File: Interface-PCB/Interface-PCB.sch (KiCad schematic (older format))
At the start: 9 parts, among them J1 BARREL_JACK_PAD, J2 BARREL_JACK_PAD, J3 RASPBERRYPI-40-PIN-GPIO, J4 I2C_HEADER, M1 PERISTALTIC_PUMP, M2 PERISTALTIC_PUMP, M3 PERISTALTIC_PUMP, U1 TB6612FNG_BREAKOUT, U2 TB6612FNG_BREAKOUT

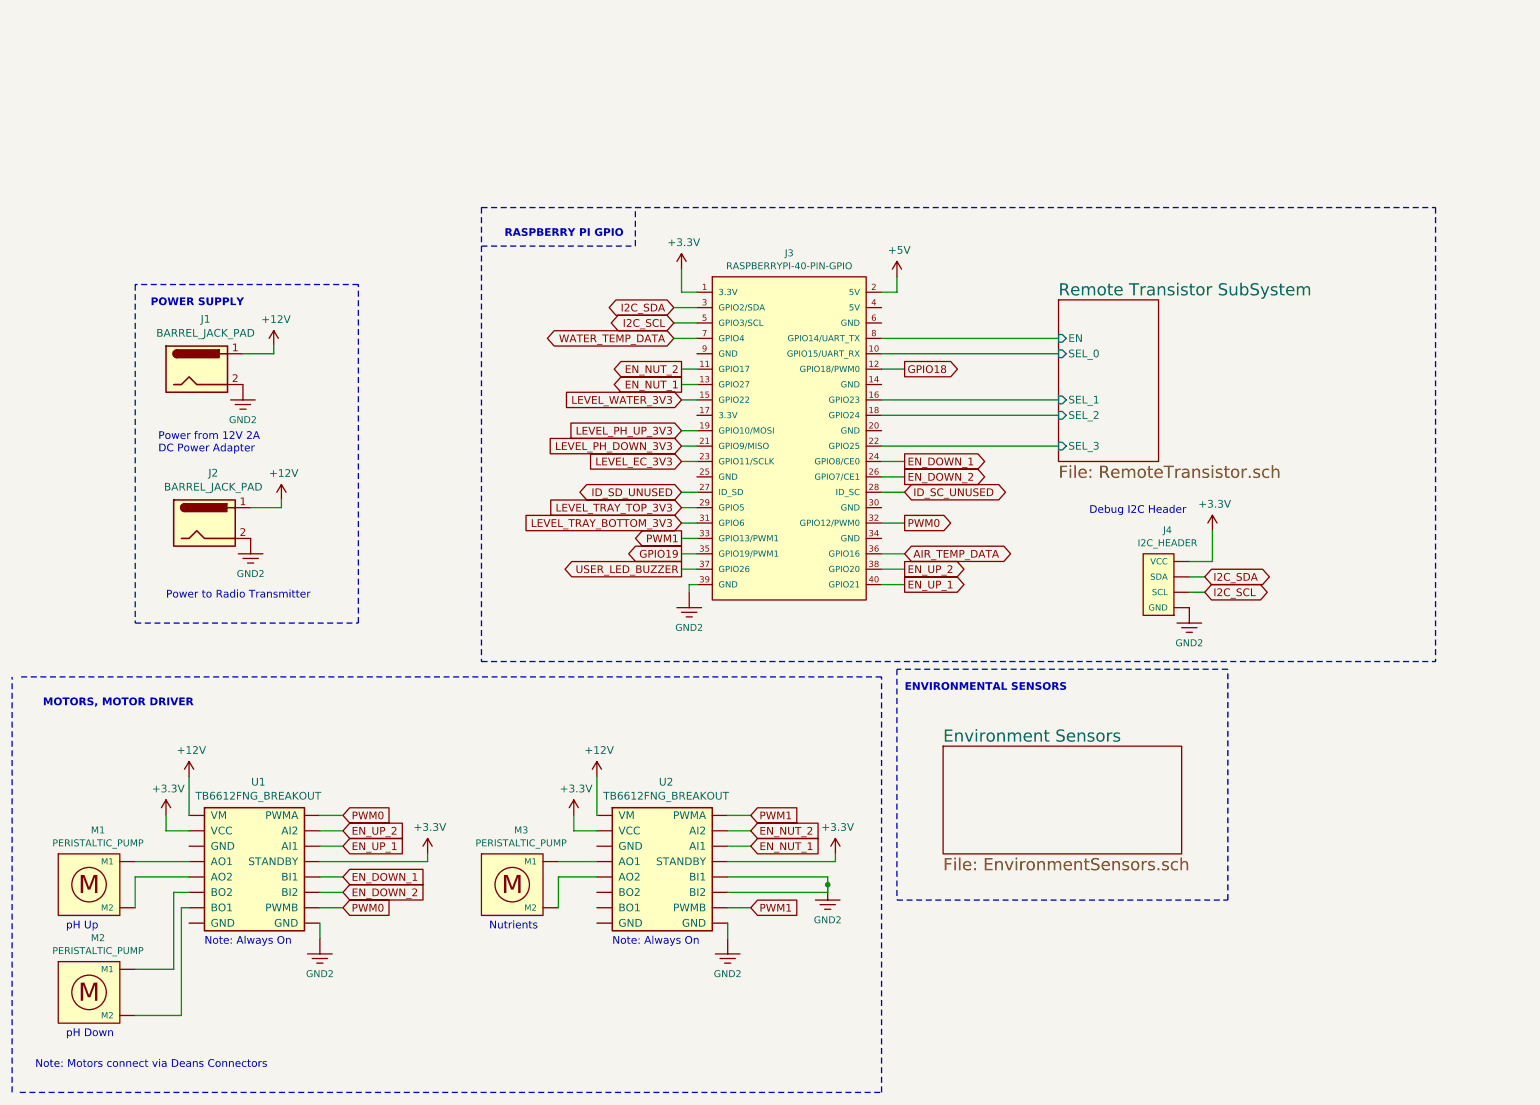
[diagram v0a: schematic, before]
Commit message: Review Schematic
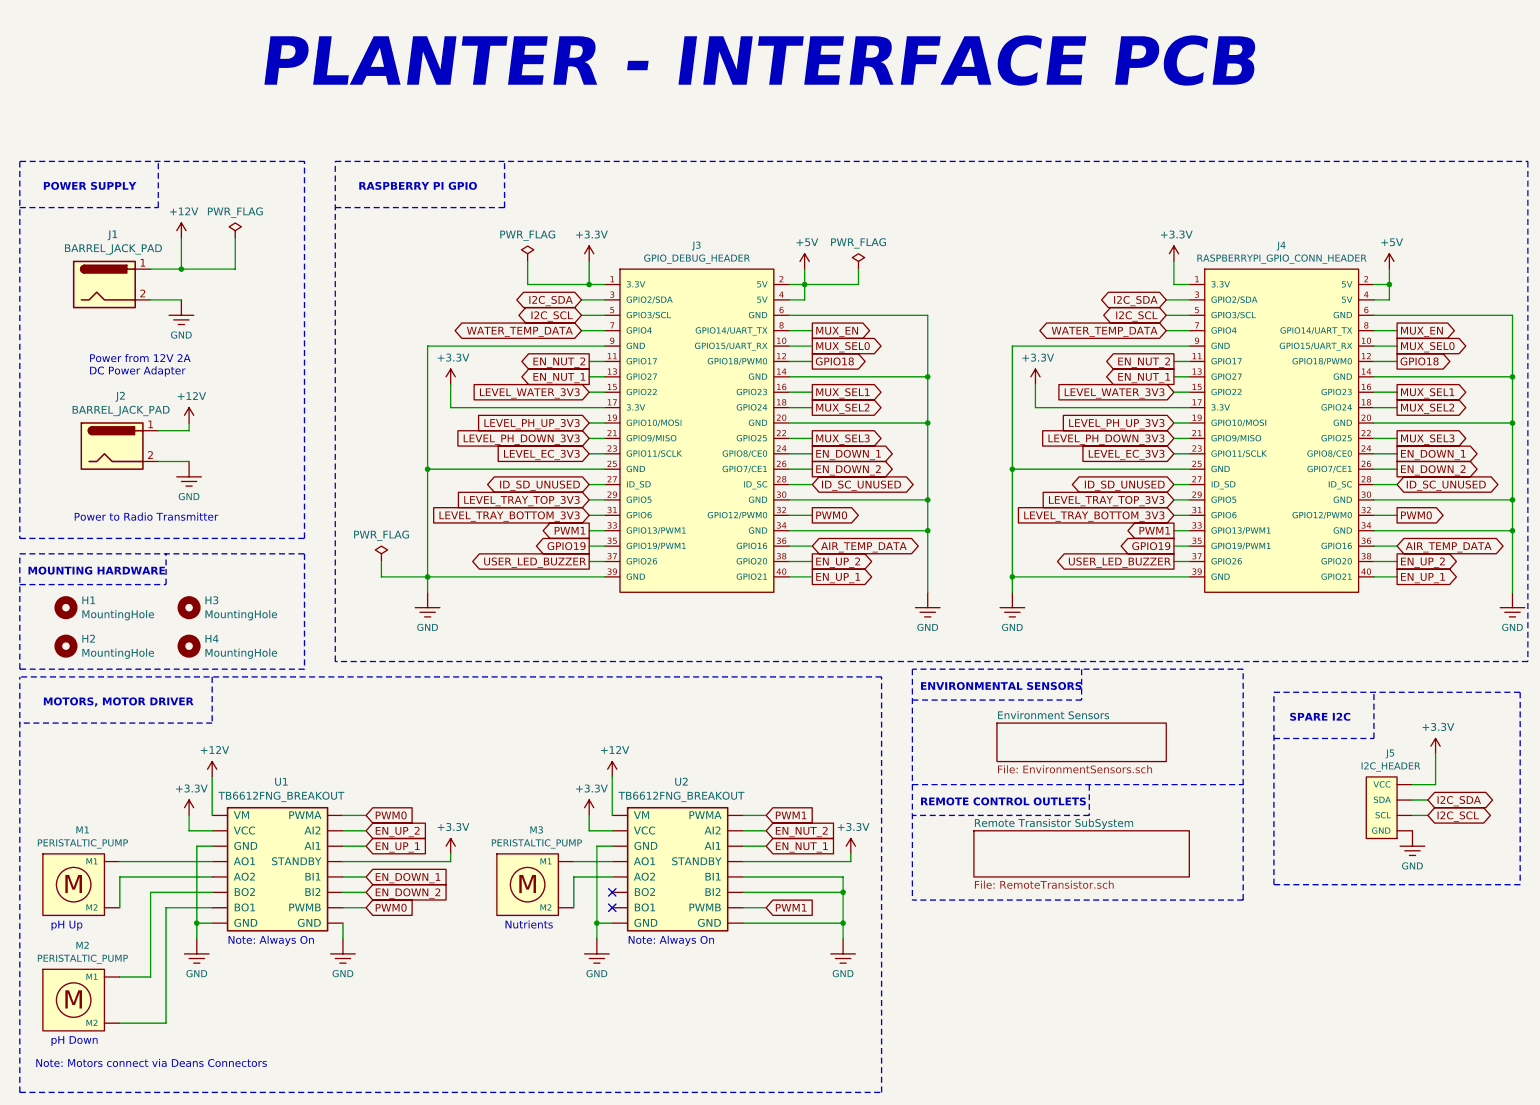
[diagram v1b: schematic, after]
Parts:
- added H1, H2, H3, H4: MountingHole, MountingHole:MountingHole_3.2mm_M3_Pad, symbol Mechanical:MountingHole
- added J3: GPIO_DEBUG_HEADER, Connector_PinHeader_2.54mm:PinHeader_2x21_P2.54mm_Vertical, symbol AA_Custom_Components:RASPBERRYPI-40-PIN-GPIO
- J4: renamed from J3; value RASPBERRYPI-40-PIN-GPIO -> RASPBERRYPI_GPIO_CONN_HEADER
- U1: footprint Package_DIP:DIP-16_W7.62mm_LongPads -> digikey-footprints:DIP-16_W7.62mm
- renumbered J4 to J5
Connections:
- net 3.3V is gone; now on net GND: J1.2, J2.2, J4.39 (GND), J5.4 (GND), U1.16 (GND), U2.13 (BI1), U2.14 (BI2), U2.16 (GND)
- net +3V3: now also J4.17 (3.3V), J3.1 (3.3V), J3.17 (3.3V)
- net +5V: now also J4.4 (5V), J3.2 (5V), J3.4 (5V)
- net AIR_TEMP_DATA: now also J3.36 (GPIO16)
- net EN_DOWN_1: now also J3.24 (GPIO8/CE0)
- net EN_DOWN_2: now also J3.26 (GPIO7/CE1)
- net EN_NUT_1: now also J3.13 (GPIO27)
- net EN_NUT_2: now also J3.11 (GPIO17)
- net EN_UP_1: now also J3.40 (GPIO21)
- net EN_UP_2: now also J3.38 (GPIO20)
- net GPIO18: now also J3.12 (GPIO18/PWM0)
- net GPIO19: now also J3.35 (GPIO19/PWM1)
- net I2C_SCL: now also J3.5 (GPIO3/SCL)
- net I2C_SDA: now also J3.3 (GPIO2/SDA)
- net ID_SC_UNUSED: now also J3.28 (ID_SC)
- net ID_SD_UNUSED: now also J3.27 (ID_SD)
- net LEVEL_EC_3V3: now also J3.23 (GPIO11/SCLK)
- net LEVEL_PH_DOWN_3V3: now also J3.21 (GPIO9/MISO)
- net LEVEL_PH_UP_3V3: now also J3.19 (GPIO10/MOSI)
- net LEVEL_TRAY_BOTTOM_3V3: now also J3.31 (GPIO6)
- net LEVEL_TRAY_TOP_3V3: now also J3.29 (GPIO5)
- net LEVEL_WATER_3V3: now also J3.15 (GPIO22)
- net PWM0: now also J3.32 (GPIO12/PWM0)
- net PWM1: now also J3.33 (GPIO13/PWM1)
- net USER_LED_BUZZER: now also J3.37 (GPIO26)
- net WATER_TEMP_DATA: now also J3.7 (GPIO4)
- net GND: now reaches J4.14 (GND)
- net GND: now also J4.20 (GND), J4.25 (GND), J4.30 (GND), J4.34 (GND), J4.6 (GND), J4.9 (GND), U1.3 (GND), U1.8 (GND), U2.3 (GND), U2.8 (GND), J3.14 (GND), J3.20 (GND), J3.25 (GND), J3.30 (GND), J3.34 (GND), J3.39 (GND), J3.6 (GND), J3.9 (GND)
- net Remote Transistor SubSystem/EN renamed MUX_EN
- net MUX_EN: now also J3.8 (GPIO14/UART_TX)
- net Remote Transistor SubSystem/SEL_0 renamed MUX_SEL0
- net MUX_SEL0: now also J3.10 (GPIO15/UART_RX)
- net Remote Transistor SubSystem/SEL_1 renamed MUX_SEL1
- net MUX_SEL1: now also J3.16 (GPIO23)
- net Remote Transistor SubSystem/SEL_2 renamed MUX_SEL2
- net MUX_SEL2: now also J3.18 (GPIO24)
- net Remote Transistor SubSystem/SEL_3 renamed MUX_SEL3
- net MUX_SEL3: now also J3.22 (GPIO25)
- no-connect marks 0 -> 2
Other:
- note added: "MOUNTING HARDWARE"
- note added: "PLANTER - INTERFACE PCB"
- note added: "REMOTE CONTROL OUTLETS"
- note added: "SPARE I2C"
- note removed: "Debug I2C Header"
- moved on the sheet: J1, J2, J4, J5, M1, M2, M3, U1, U2
